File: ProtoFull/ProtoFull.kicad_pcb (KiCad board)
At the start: 2 copper layers, 111.8 x 68.6 mm, 77 parts, among them J1 AVR-ISP-6, Q1 BSS138, SW1 SW_Push, SW2 RotaryEncoder_Switch, SW3 RotaryEncoder_Switch, U1 PRTR5V0U2X, U2 AT90USB1286-AU, U3 UG-2864HSWEG01, U4 AP2112K-3.3, X1 IS31FL3741, Y1 16MHz

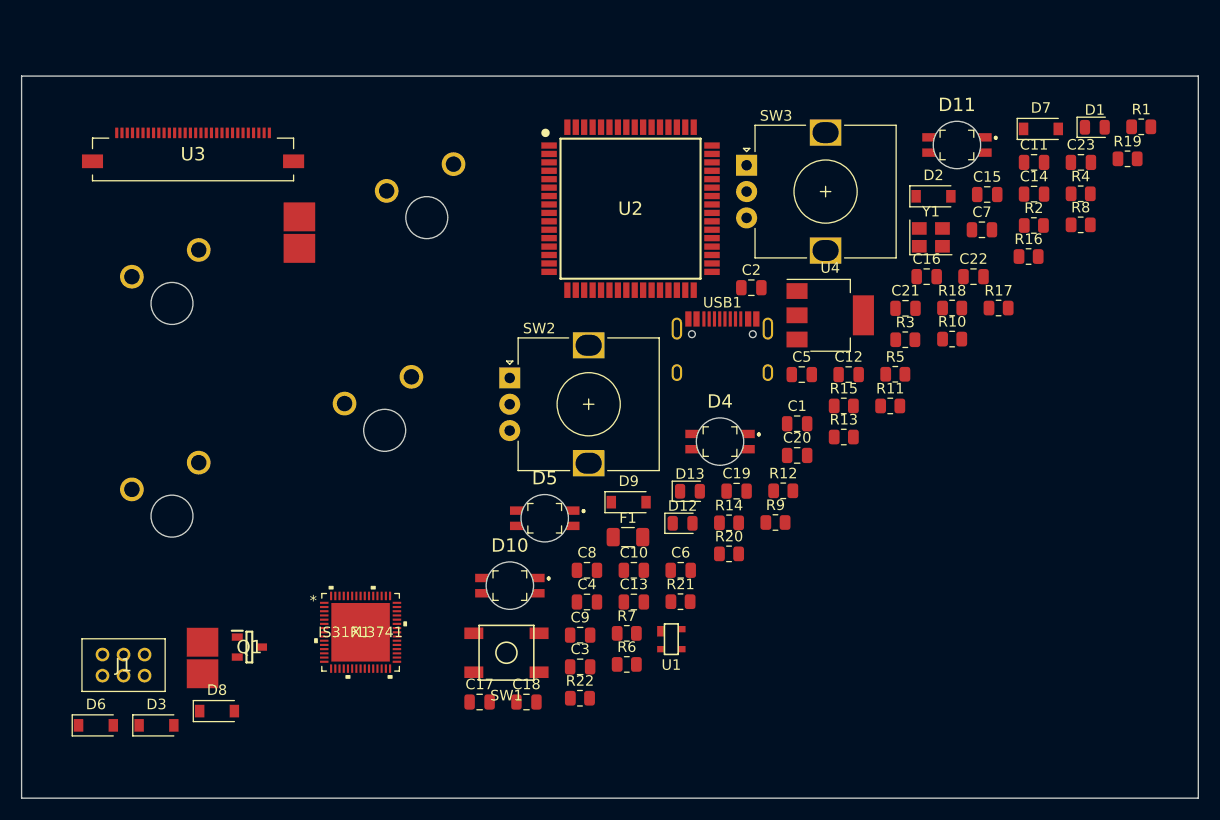
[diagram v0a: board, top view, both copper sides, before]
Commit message: Merge Schematics, OLED not sure
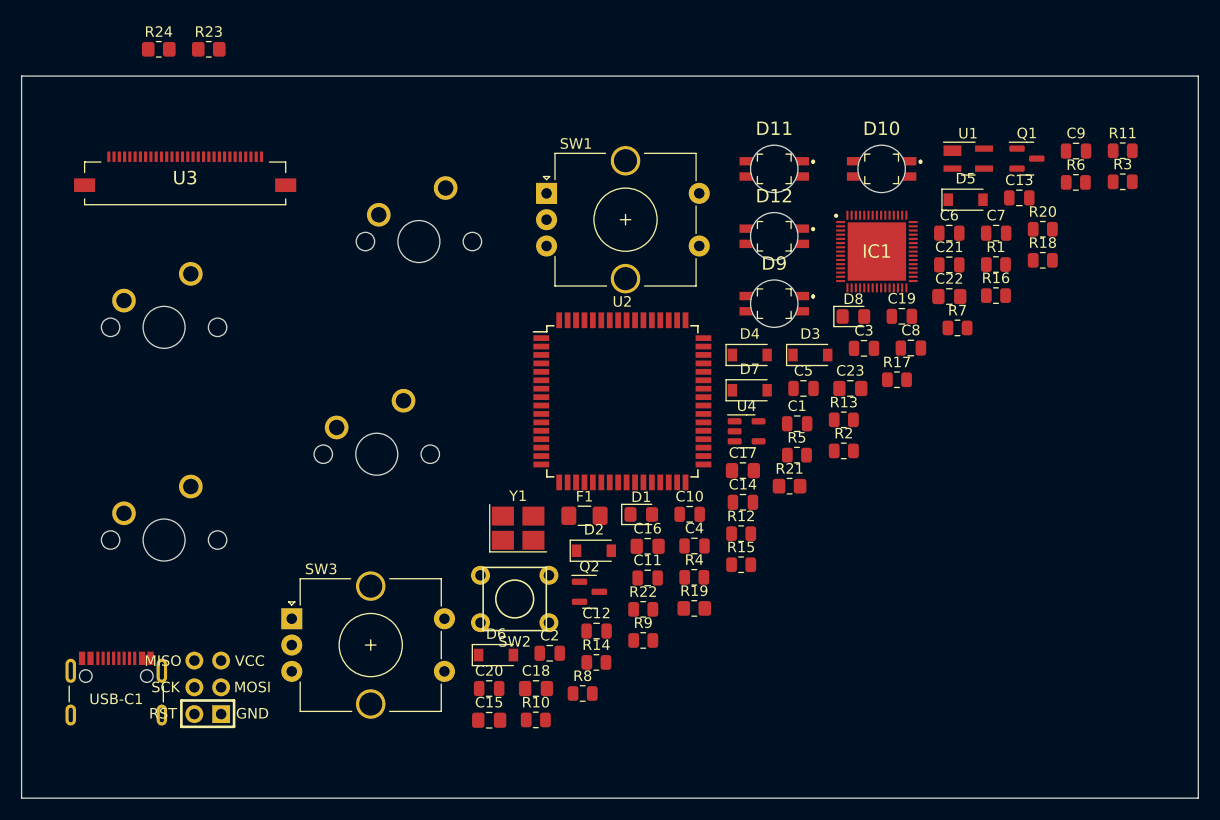
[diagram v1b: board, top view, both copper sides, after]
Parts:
- removed D13: GREEN, LED_SMD:LED_0805_2012Metric
- removed SJ1: SOLDERJUMPER, random-keyboard-parts:Jumper-UserFriendly
- removed SJ2: SOLDERJUMPERCLOSED, random-keyboard-parts:Jumper-UserFriendly
- removed USB1: HRO-TYPE-C-31-M-12, Type-C:HRO-TYPE-C-31-M-12
- removed X1: IS31FL3741, Breadboard:IS31FL3741-QFLS4-TR
- added IC1: IS31FL3741, SamacSys_Parts:QFN40P700X700X80-61N-D, F.Cu at (165.1, 62.4)
- added Q2: BSS138, Package_TO_SOT_SMD:SOT-23, F.Cu at (137.8, 94.7)
- added R23: 10k, Resistor_SMD:R_0805_2012Metric_Pad1.20x1.40mm_HandSolder, F.Cu at (101.6, 43.2)
- added R24: 390k, Resistor_SMD:R_0805_2012Metric_Pad1.20x1.40mm_HandSolder, F.Cu at (96.8, 43.2)
- added USB-C1: HRO-TYPE-C-31-M-12, SamacSys_Parts:TYPE-C-31-M-12, F.Cu at (92.8, 106.4)
- C10, C8: value 1uF -> 0.1uF
- C11, C19: value 10uF -> 1uF
- C13: value 0.1uF -> 1uF
- C15, C16: value 2.2uF -> 1uF; footprint Capacitor_SMD:C_0805_2012Metric -> Capacitor_SMD:C_0805_2012Metric_Pad1.18x1.45mm_HandSolder
- C17: value 1uF -> 0.1uF; footprint Capacitor_SMD:C_0805_2012Metric -> Capacitor_SMD:C_0805_2012Metric_Pad1.18x1.45mm_HandSolder
- C18: value 10uF -> 1uF; footprint Capacitor_SMD:C_0805_2012Metric -> Capacitor_SMD:C_0805_2012Metric_Pad1.18x1.45mm_HandSolder
- C20, C5, C9: value 10uF -> 0.1uF
- C22: value 10uF -> 4,7uF 16V; footprint Capacitor_SMD:C_0805_2012Metric -> Capacitor_SMD:C_0805_2012Metric_Pad1.18x1.45mm_HandSolder
- C23: value 10uF -> 2,2uF; footprint Capacitor_SMD:C_0805_2012Metric -> Capacitor_SMD:C_0805_2012Metric_Pad1.18x1.45mm_HandSolder
- C3: value 1uF -> 10uF
- C4: value 22pF -> 10uF
- C6: value 10uF -> 22pF
- D1: footprint LED_SMD:LED_0805_2012Metric -> LED_SMD:LED_0805_2012Metric_Pad1.15x1.40mm_HandSolder
- D12: value LED_YELLOW -> LED_BGRA; footprint LED_SMD:LED_0805_2012Metric -> SamacSys_Parts:QBLP677R-RGB
- D2, D3, D6, D7: value SOD-123 -> 1N4148W
- D4, D5: value LED_BGRA -> 1N4148W; footprint SamacSys_Parts:QBLP677R-RGB -> Diode_SMD:D_SOD-123
- D8: value SOD-123 -> GREEN; footprint Diode_SMD:D_SOD-123 -> LED_SMD:LED_0805_2012Metric_Pad1.15x1.40mm_HandSolder
- D9: value SOD-123 -> LED_BGRA; footprint Diode_SMD:D_SOD-123 -> SamacSys_Parts:QBLP677R-RGB
- F1: footprint Fuse:Fuse_1206_3216Metric -> Fuse:Fuse_1206_3216Metric_Pad1.42x1.75mm_HandSolder
- J1: footprint SamacSys_Parts:SWR204NRTND03STGA -> random-keyboard-parts:Reset_Pretty
- MX1, MX2, MX3, MX4: footprint SamacSys_Parts:MXOnly-1U-NoLED_3Pins -> MX_Only:MXOnly-1U-NoLED
- Q1: footprint SamacSys_Parts:SOT95P240X120-3N -> Package_TO_SOT_SMD:SOT-23
- R1: value 200 -> 680
- R10, R11: value 22 -> 10k
- R12: value 51 -> 10k
- R16: value 100K -> 22
- R17: value 10K -> 22
- R18: value 200 -> 51
- R19: value 10K -> 10k; footprint Resistor_SMD:R_0805_2012Metric -> Resistor_SMD:R_0805_2012Metric_Pad1.20x1.40mm_HandSolder
- R20, R22: value 10K -> 10k
- R21: value 390K -> 10k; footprint Resistor_SMD:R_0805_2012Metric -> Resistor_SMD:R_0805_2012Metric_Pad1.20x1.40mm_HandSolder
- R8: value 4.7K -> 270
- R9: value 4.7K -> 10k
- SW1: value SW_Push -> RotaryEncoder_Switch; footprint random-keyboard-parts:SKQG-1155865 -> Rotary_Encoder:RotaryEncoder_Alps_EC12E-Switch_Vertical_H20mm_CircularMountingHoles
- SW2: value RotaryEncoder_Switch -> RESET; footprint Rotary_Encoder:RotaryEncoder_Alps_EC12E_Vertical_H20mm -> random-keyboard-parts:PushButton_6x6mm_TH
- SW3: footprint Rotary_Encoder:RotaryEncoder_Alps_EC12E_Vertical_H20mm -> Rotary_Encoder:RotaryEncoder_Alps_EC12E-Switch_Vertical_H20mm_CircularMountingHoles
- U1: footprint random-keyboard-parts:SOT143B -> Package_TO_SOT_SMD:SOT-143_Handsoldering
- U2: value AT90USB1286-AU -> AT90USB1286-A; footprint SamacSys_Parts:AT90USB1286-AU -> Package_QFP:TQFP-64_14x14mm_P0.8mm
- U4: footprint Package_TO_SOT_SMD:SOT-223-3_TabPin2 -> Package_TO_SOT_SMD:SOT-23-5
- Y1: footprint Crystal:Crystal_SMD_3225-4Pin_3.2x2.5mm -> Crystal:Crystal_SMD_3225-4Pin_3.2x2.5mm_HandSoldering
- moved Q1 87.2 mm to (179.3, 53.6)
- moved D3 71.4 mm to (158.7, 72.2)
- moved D8 71.1 mm to (162.8, 68.6)
- moved C15 68.8 mm to (128.2, 106.9)
- moved C9 65.8 mm to (184.0, 52.8)
- moved R8 64.9 mm to (137.1, 104.4)
- moved R6 62.6 mm to (183.9, 55.8)
- moved SW3 61.0 mm to (109.5, 97.3)
- moved R19 59.3 mm to (147.7, 96.3)
- moved D1 56.6 mm to (142.7, 87.4)
- moved C11 53.9 mm to (143.3, 93.4)
- moved U1 53.6 mm to (173.7, 53.6)
- moved R10 53.6 mm to (132.7, 106.9)
- moved D10 53.0 mm to (165.5, 54.5)
- moved C13 53.0 mm to (178.6, 57.3)
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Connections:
- C10 pad 1: VCC -> +5V
- C11 pad 1: GND -> +5V
- C11 pad 2: +5V -> GND
- C12 pad 1: GND -> +5V
- C12 pad 2: +5V -> GND
- C13 pad 1: GND -> +5V
- C13 pad 2: +5V -> GND
- C14 pad 1: GND -> +5V
- C14 pad 2: +5V -> GND
- C15 pad 1: Net-(C15-Pad1) -> GND
- C15 pad 2: Net-(C15-Pad2) -> +3V3
- C16 pad 1: Net-(C16-Pad1) -> /C2P
- C16 pad 2: Net-(C16-Pad2) -> /C2N
- C17 pad 2: 3.3V -> +3V3
- C18 pad 1: GND -> /C1P
- C18 pad 2: 3.3V -> /C1N
- C20 pad 1: 3.3V -> +5V
- C21 pad 1: 3.3V -> Net-(C21-Pad1)
- C22 pad 1: GND -> /VCOMH
- C22 pad 2: Net-(C22-Pad2) -> GND
- C23 pad 1: GND -> VCC
- C23 pad 2: Net-(C23-Pad2) -> GND
- C3 pad 1: VCC -> +5V
- C3 pad 2: Net-(C3-Pad2) -> GND
- C4 pad 1: GND -> +3V3
- C4 pad 2: XTAL2 -> GND
- C5 pad 1: VCC -> +3V3
- C6 pad 1: VCC -> GND
- C6 pad 2: GND -> XTAL2
- C7 pad 1: VCC -> +5V
- C8 pad 1: VCC -> +5V
- C9 pad 1: VCC -> +5V
- D10 pad 1: CS4_B -> CS1_B
- D10 pad 2: CS5_G -> CS2_G
- D10 pad 3: CS6_R -> CS3_R
- D10 pad 4: SW1 -> SW2
- D11 pad 4: SW2 -> SW1
- D12 pad 1: GND -> CS4_B
- D12 pad 2: Net-(D12-Pad2) -> CS5_G
- D2 pad 1: ROT1_ROW -> ROW0
- D3 pad 1: ROT2_ROW -> ROW0
- D4 pad 1: CS1_B -> ROW0
- D4 pad 2: CS2_G -> Net-(D4-Pad2)
- D5 pad 1: CS1_B -> ROW1
- D5 pad 2: CS2_G -> Net-(D5-Pad2)
- D6 pad 1: ROT1_ROW -> ROW1
- D7 pad 1: ROT1_ROW -> ROW1
- D8 pad 1: ROT2_ROW -> GND
- D9 pad 1: ROT2_ROW -> CS1_B
- D9 pad 2: Net-(D9-Pad2) -> CS2_G
- F1 pad 1: +5V -> VCC
- F1 pad 2: VCC -> +5V
- J1 pad 2: +5V -> VCC
- MX1 pad 2: Net-(D6-Pad2) -> Net-(D2-Pad2)
- MX2 pad 2: Net-(D7-Pad2) -> Net-(D3-Pad2)
- MX3 pad 2: Net-(D8-Pad2) -> Net-(D5-Pad2)
- MX4 pad 2: Net-(D9-Pad2) -> Net-(D6-Pad2)
- Q1 pad 1: SCL_3.3 -> +3V3
- Q1 pad 2: 3.3V -> SDA_3.3
- R1 pad 1: Net-(D1-Pad2) -> VCC
- R1 pad 2: VCC -> Net-(D1-Pad2)
- R10 pad 1: Net-(R10-Pad1) -> +5V
- R10 pad 2: CS1_B -> SDA
- R11 pad 1: Net-(R11-Pad1) -> +3V3
- R11 pad 2: CS2_G -> SCL_3.3
- R12 pad 1: Net-(R12-Pad1) -> +3V3
- R12 pad 2: CS3_R -> SDA_3.3
- R13 pad 2: CS4_B -> CS1_B
- R14 pad 2: CS5_G -> CS2_G
- R15 pad 2: CS6_R -> CS3_R
- R16 pad 1: Net-(C3-Pad2) -> Net-(IC1-Pad29)
- R16 pad 2: Net-(R16-Pad2) -> CS4_B
- R17 pad 1: GND -> Net-(IC1-Pad30)
- R17 pad 2: Net-(R17-Pad2) -> CS5_G
- R18 pad 1: Net-(D12-Pad2) -> Net-(IC1-Pad31)
- R18 pad 2: +5V -> CS6_R
- R19 pad 1: GND -> /BS0
- R19 pad 2: 3.3V -> GND
- R20 pad 2: (no net) -> Net-(C21-Pad1)
- R21 pad 1: GND -> /BS1
- R21 pad 2: Net-(R21-Pad2) -> GND
- R3 pad 1: D- -> Net-(R3-Pad1)
- R3 pad 2: Net-(R3-Pad2) -> D-
- R4 pad 1: D+ -> Net-(R4-Pad1)
- R4 pad 2: Net-(R4-Pad2) -> D+
- R7 pad 1: Net-(R7-Pad1) -> GND
- R7 pad 2: GND -> Net-(R7-Pad2)
- R8 pad 1: SCL -> +3V3
- R8 pad 2: VCC -> Net-(D8-Pad2)
- R9 pad 1: SDA -> +5V
- R9 pad 2: VCC -> SCL
- U1 pad 2: Net-(R4-Pad2) -> Net-(R4-Pad1)
- U1 pad 3: Net-(R3-Pad2) -> Net-(R3-Pad1)
- U2 pad 33: ROT2_ROW -> ROW1
- U2 pad 34: ROT1_ROW -> ROW0
- U2 pad 43: Net-(R7-Pad1) -> Net-(R7-Pad2)
- U3 pad 10: GND -> /BS0
- U3 pad 11: 3.3V -> /BS1
- U3 pad 12: GND -> /BS2
- U3 pad 13: unconnected-(U3-Pad13) -> GND
- U3 pad 2: Net-(C15-Pad2) -> /C2P
- U3 pad 20: Net-(SJ2-Pad2) -> /D2/SDA
- U3 pad 26: Net-(R21-Pad2) -> /IREF
- U3 pad 27: Net-(C22-Pad2) -> /VCOMH
- U3 pad 28: Net-(C23-Pad2) -> VCC
- U3 pad 3: Net-(C15-Pad1) -> /C2N
- U3 pad 4: Net-(C16-Pad2) -> /C1P
- U3 pad 5: Net-(C16-Pad1) -> /C1N
- U3 pad 6: 3.3V -> +3V3
- U3 pad 9: 3.3V -> +3V3
